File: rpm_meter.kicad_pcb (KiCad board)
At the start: 2 copper layers, 153.8 x 95.2 mm, 112 parts, among them IC1 SN74LV1T34DCKR, IC6 TPS566247DRLR, J1 Conn_01x01_Socket, J2 Conn_2Rows-05Pins, J3 Conn_01x01_Socket, J4 Conn_01x01_Socket, J5 Conn_01x01_Socket, J6 Conn_01x01_Socket, J7 Conn_01x01_Socket, Q1 BC846, Q14 BC846, Q15 BC846, Q16 BC846, U1 M24C02-RMN, U2 STM32C031C6Tx, U3 74LVC1G123, U4 TLV1117-33, U5 PEC11R-4225F-S0024, Y1 8

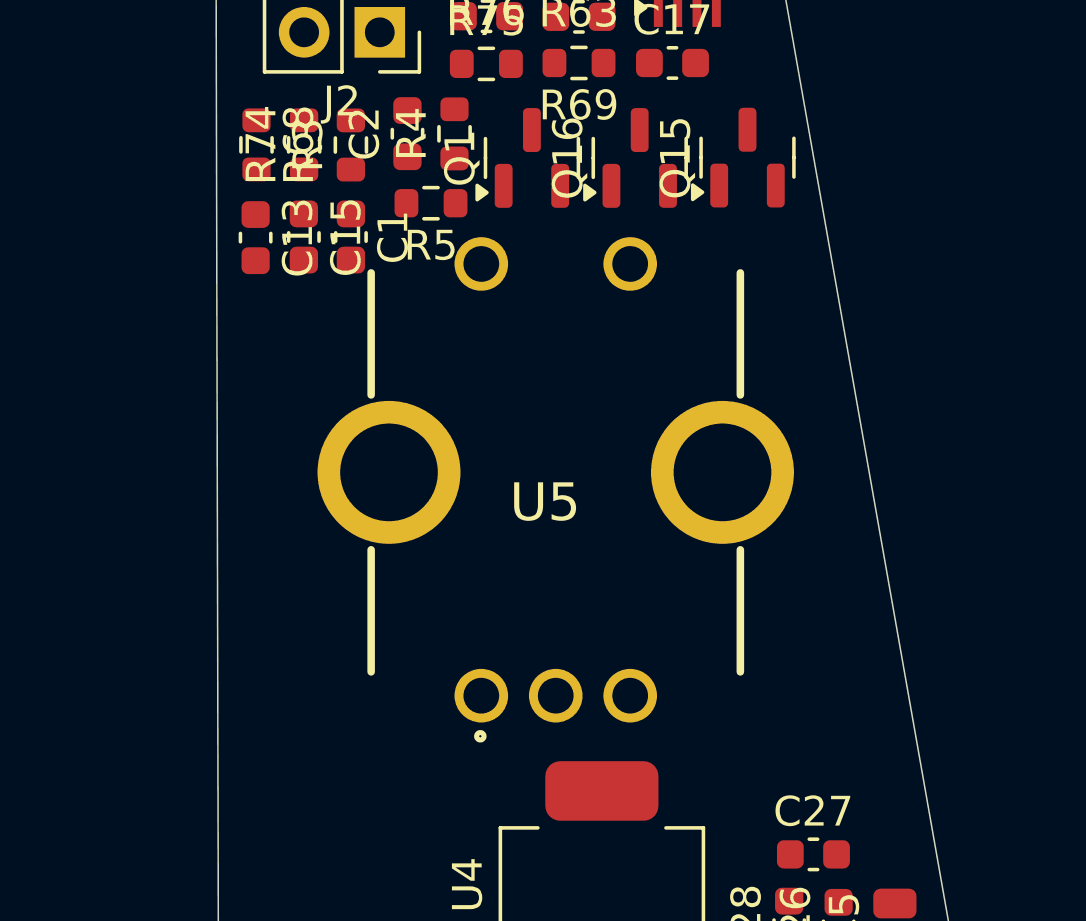
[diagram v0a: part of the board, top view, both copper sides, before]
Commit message: Encoder
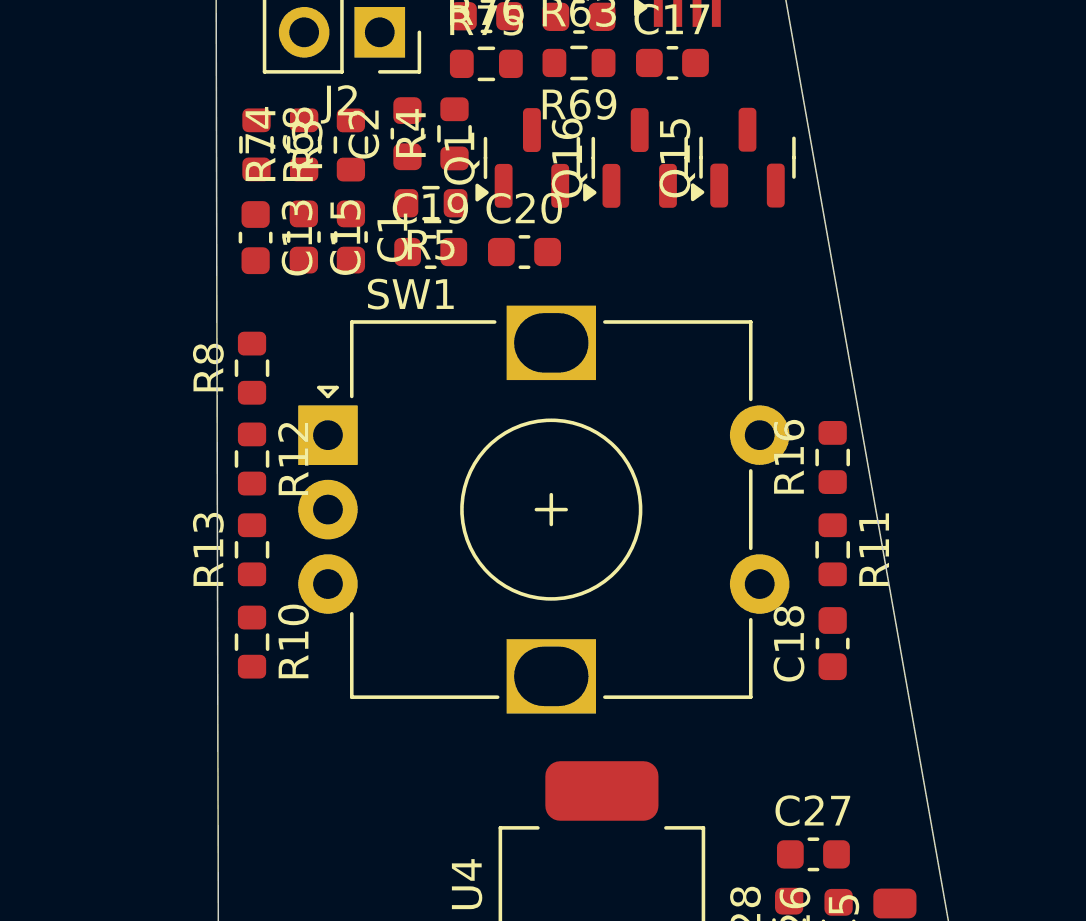
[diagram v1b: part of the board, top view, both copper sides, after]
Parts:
- removed U5: PEC11R-4225F-S0024, Library_local:PEC12R-4XXXF-SXXXX_1
- added C18: 100n, Capacitor_SMD:C_0603_1608Metric, F.Cu at (214.6, 89.7)
- added C19: 100n, Capacitor_SMD:C_0603_1608Metric, F.Cu at (201.1, 76.5)
- added C20: 100n, Capacitor_SMD:C_0603_1608Metric, F.Cu at (204.2, 76.5)
- added R10: 10k, Resistor_SMD:R_0603_1608Metric, F.Cu at (195.1, 89.6)
- added R11: 10k, Resistor_SMD:R_0603_1608Metric, F.Cu at (214.6, 86.5)
- added R12: 1k, Resistor_SMD:R_0603_1608Metric, F.Cu at (195.1, 83.5)
- added R13: 1k, Resistor_SMD:R_0603_1608Metric, F.Cu at (195.1, 86.5)
- added R16: 1k, Resistor_SMD:R_0603_1608Metric, F.Cu at (214.6, 83.4)
- added R8: 10k, Resistor_SMD:R_0603_1608Metric, F.Cu at (195.1, 80.4)
- added SW1: RotaryEncoder_Switch_MP, Library_local:RotaryEncoder_Alps_EC12E-Switch_Vertical_H20mm, F.Cu at (197.6, 82.7)
